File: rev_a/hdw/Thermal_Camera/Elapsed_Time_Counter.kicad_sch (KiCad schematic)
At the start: 14 parts, among them J2301 I2C, J2302 UART, J2303 VOSPI, J2304 FLASH SPI

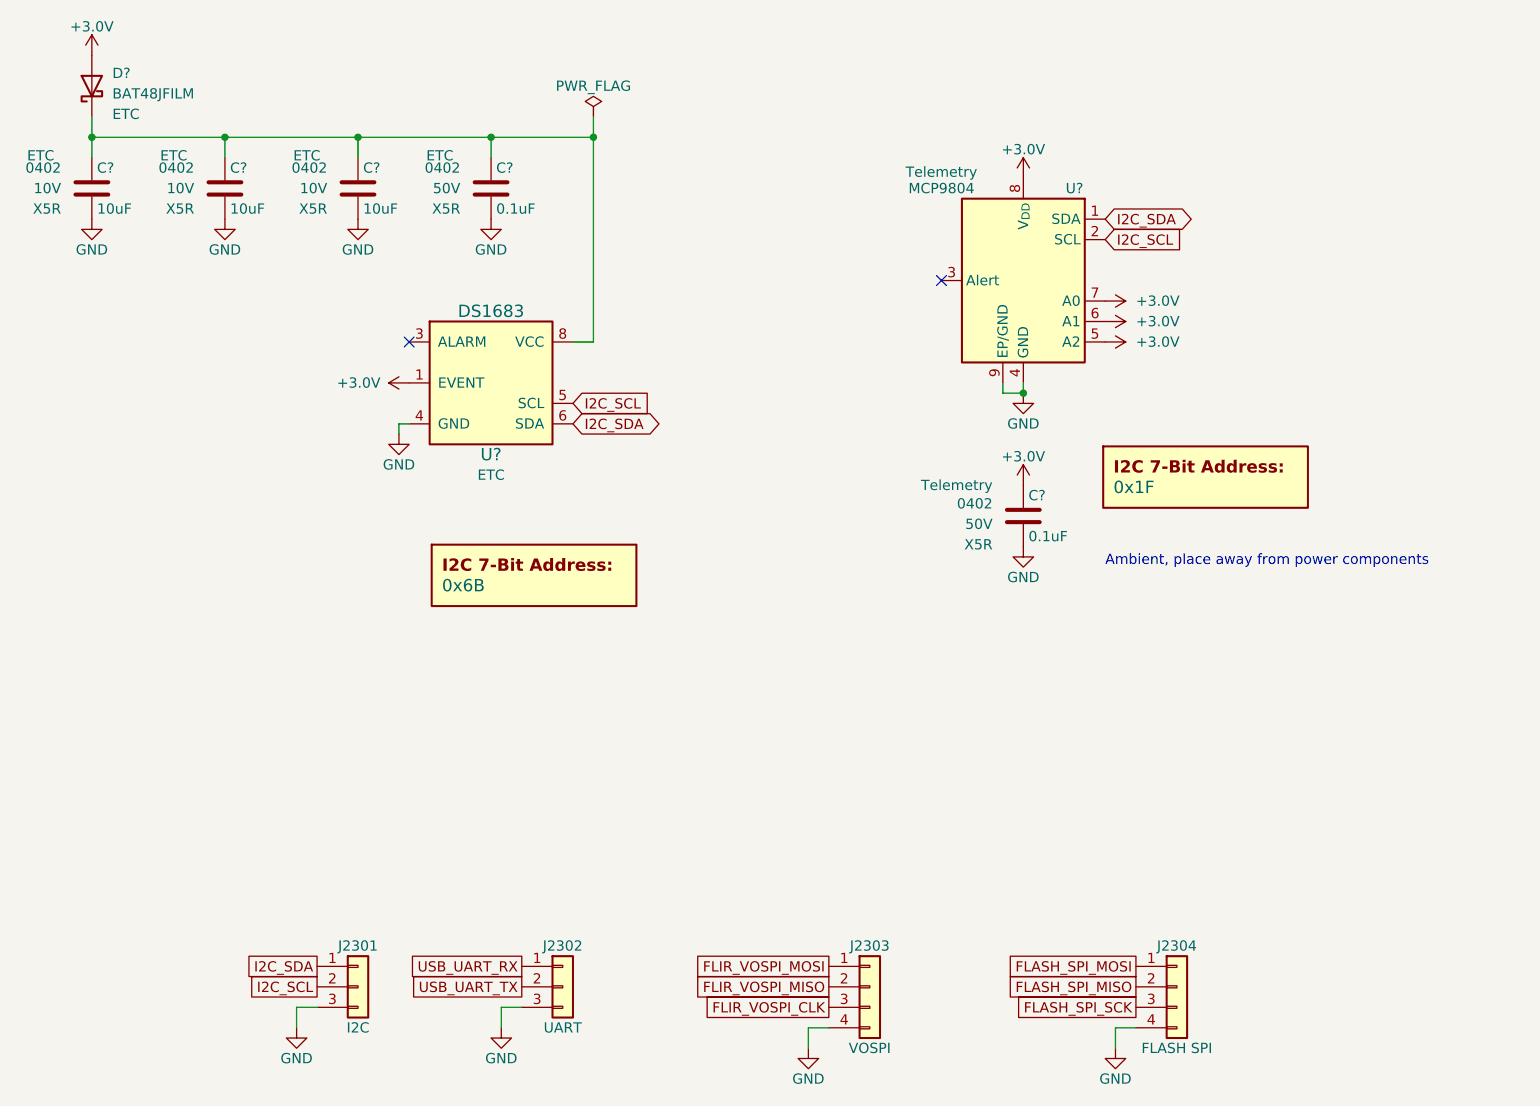
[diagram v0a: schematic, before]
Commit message: finished placing components
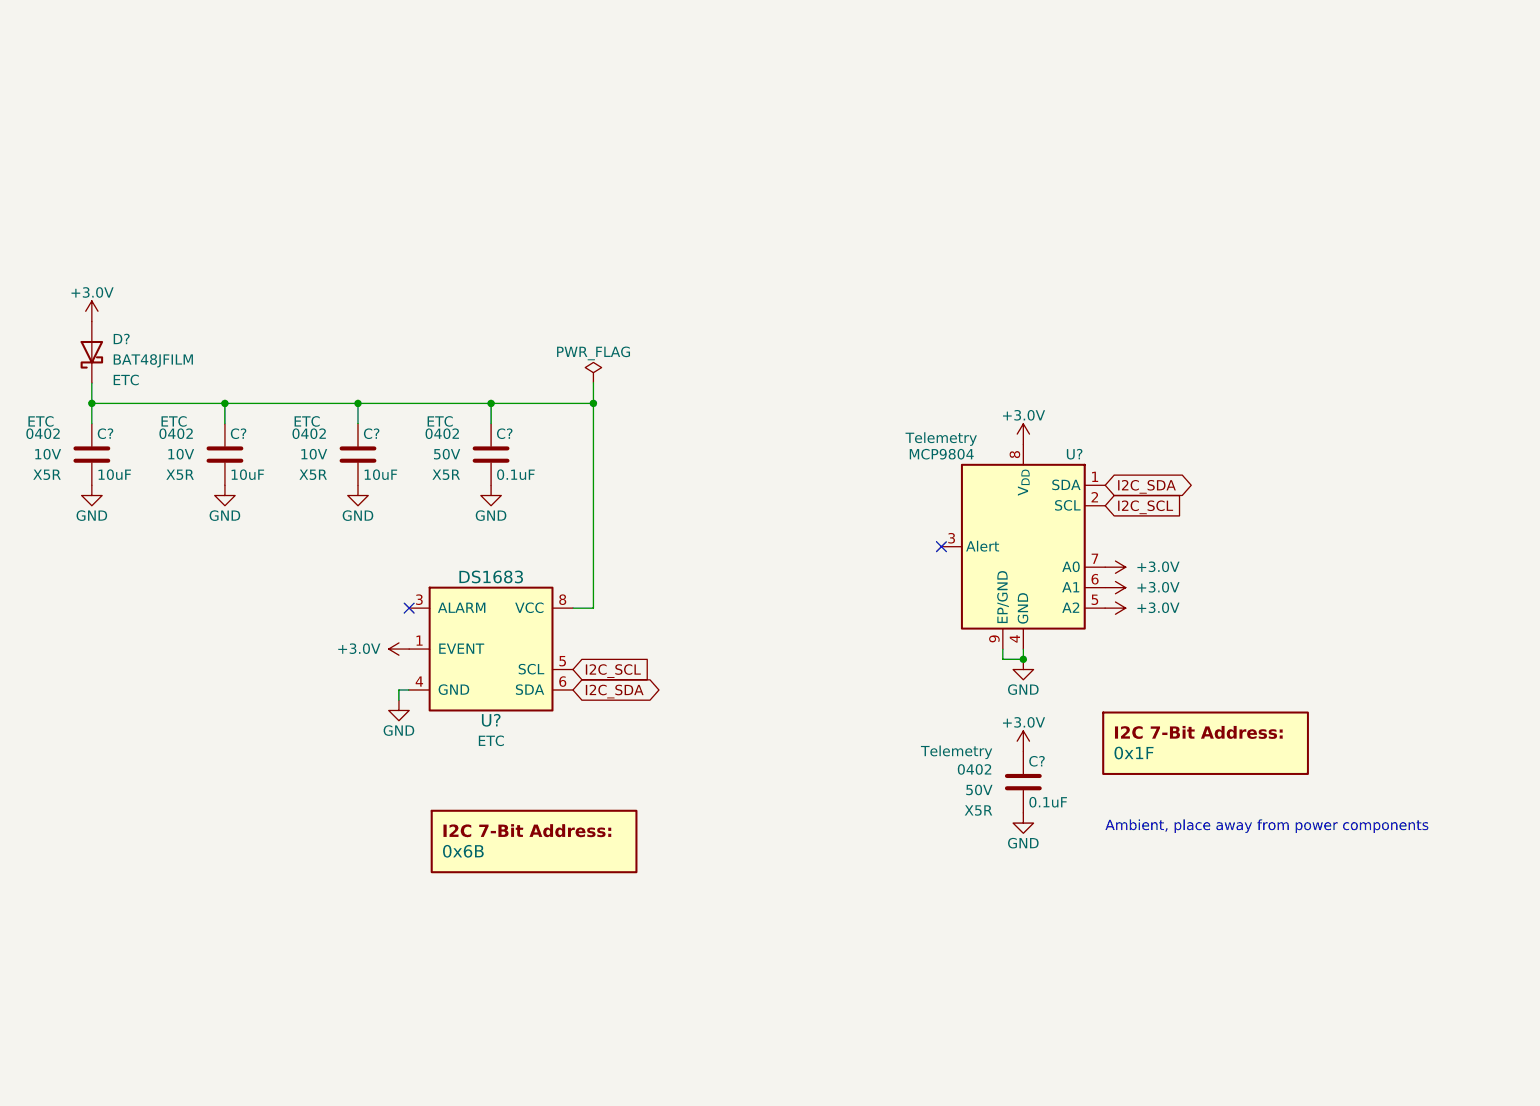
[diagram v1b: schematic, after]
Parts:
- removed J2301: I2C, Connector_PinHeader_2.54mm:PinHeader_1x03_P2.54mm_Vertical, symbol Connector_Generic:Conn_01x03
- removed J2302: UART, Connector_PinHeader_2.54mm:PinHeader_1x03_P2.54mm_Vertical, symbol Connector_Generic:Conn_01x03
- removed J2303: VOSPI, Connector_PinHeader_2.54mm:PinHeader_1x04_P2.54mm_Vertical, symbol Connector_Generic:Conn_01x04
- removed J2304: FLASH SPI, Connector_PinHeader_2.54mm:PinHeader_1x04_P2.54mm_Vertical, symbol Connector_Generic:Conn_01x04
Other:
- moved on the sheet: C?, D?, U?
